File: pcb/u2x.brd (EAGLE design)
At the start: 100 x 100 mm, 9 parts, among them IC4 REG1117, SW20 324_SW, U1 UG-2864HSWEG01, U2 CY8C5868LTI-LP039, U3 USBC_16P

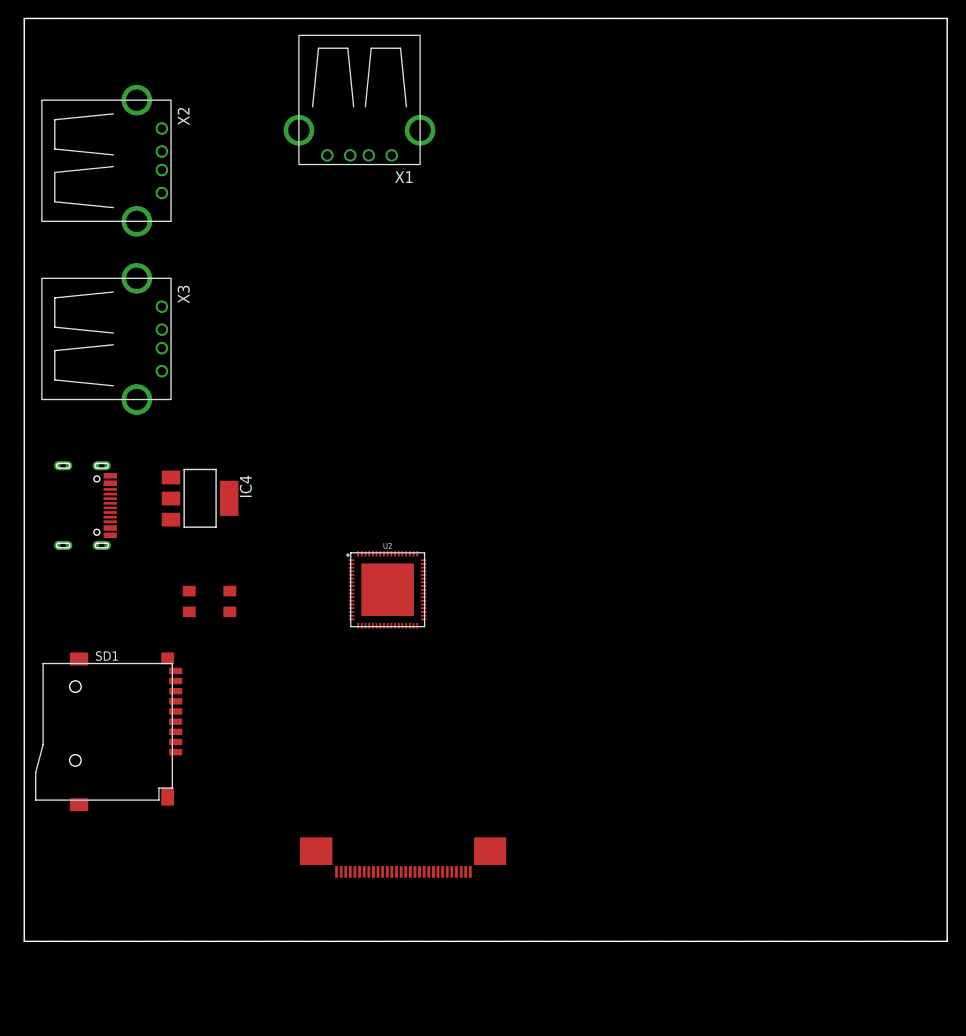
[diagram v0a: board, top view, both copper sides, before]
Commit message: started working on pcb
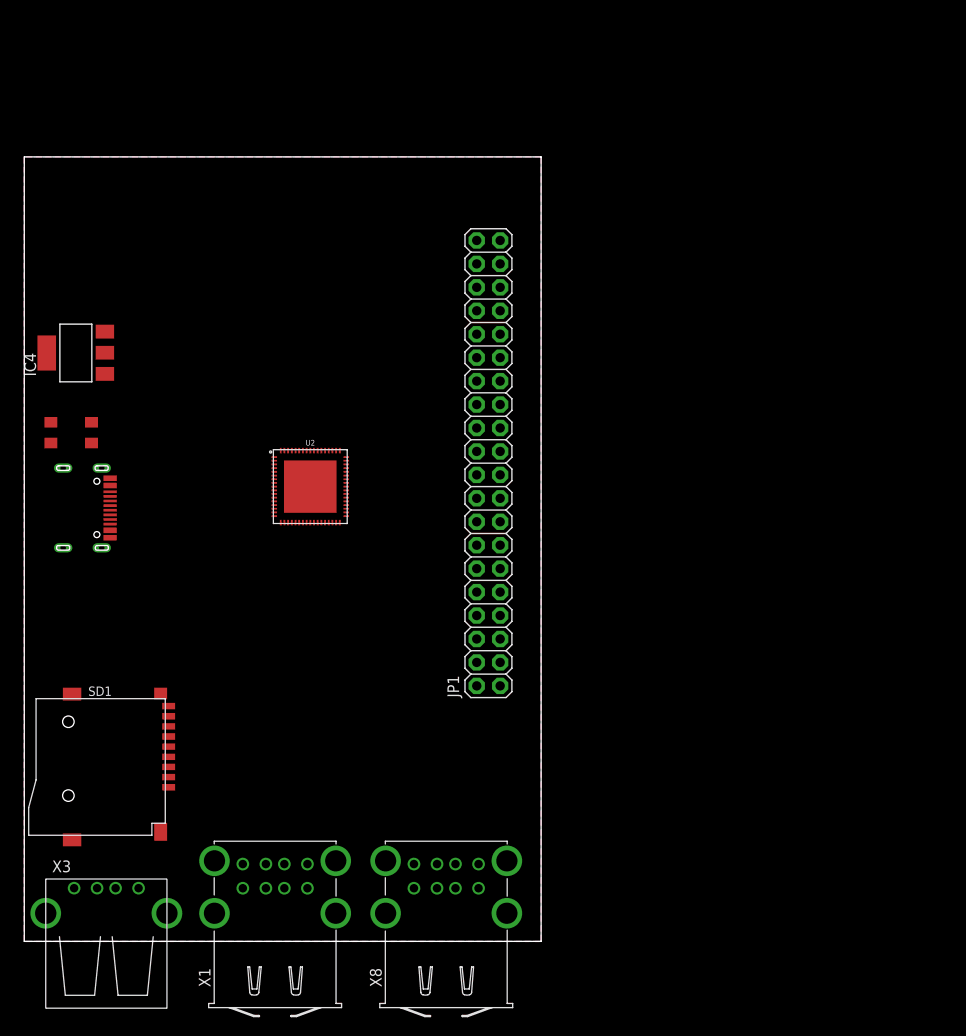
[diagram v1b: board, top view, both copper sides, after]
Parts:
- removed U1: UG-2864HSWEG01, lul:LUL_UG-2864HSWEG01_1.3_WRAPAROUND
- removed X2: (no value), bott:USB-A-H
- added JP1: (no value), adafruit_changed:2X20-BIG
- added X8: USB2, RPB:USB2
- X1: value (none) -> USB2; device bott:USB-A-H -> RPB:USB2
- moved X1 85.3 mm to (27.2, 3.05), turned to 90 degrees
- moved X3 62.3 mm to (8.89, 3.05), turned to 90 degrees
- moved SW20 23.6 mm to (5.08, 55.1)
- moved IC4 20.7 mm to (5.59, 63.8), turned to 90 degrees
- moved U2 14.0 mm to (31.0, 49.3)
- moved SD1 3.89 mm to (8.03, 18.9)
- moved U3 0.25 mm to (5.46, 47.0)
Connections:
- removed net VCC: U1.28
- removed net VLSS: U1.29
- net VDD: no longer U1.9
- net VSS: no longer U1.31, U1.32, U1.8
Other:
- board size 100 x 100 mm -> 56 x 85 mm
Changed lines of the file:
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@@
 <board>
 <plain>
-<wire x1="0" y1="100" x2="0" y2="0" width="0" layer="20"/>
-<wire x1="0" y1="0" x2="100" y2="0" width="0" layer="20"/>
-<wire x1="100" y1="0" x2="100" y2="100" width="0" layer="20"/>
-<wire x1="100" y1="100" x2="0" y2="100" width="0" layer="20"/>
-<rectangle x1="22.4834" y1="56.8782" x2="56.4834" y2="79.8782" layer="51"/>
-<rectangle x1="19.372" y1="28.992" x2="59.372" y2="43.992" layer="51" rot="R90"/>
-<rectangle x1="62.23" y1="40.894" x2="81.83" y2="65.894" layer="51"/>
+<wire x1="0" y1="85" x2="0" y2="0" width="0" layer="20"/>
+<wire x1="0" y1="0" x2="56" y2="0" width="0" layer="20"/>
+<wire x1="56" y1="0" x2="56" y2="85" width="0" layer="20"/>
+<wire x1="56" y1="85" x2="0" y2="85" width="0" layer="20"/>
 </plain>
 <attributes>
@@
 </autorouter>
 <elements>
-<element name="U3" library="my_usbc_16p" package="USBC_16P_FOOT" value="USBC_16P" x="5.461" y="47.2186" smashed="yes" rot="R270"/>
-<element name="U1" library="lul" package="LUL_UG-2864HSWEG01_1.3_WRAPAROUND" value="UG-2864HSWEG01" x="41.0784" y="7.5306" smashed="yes" rot="MR180"/>
-<element name="SD1" library="clock" package="TF-PULL" value="TF-HOLDER" x="8.7884" y="22.7076" smashed="yes" rot="R90">
-<attribute name="NAME" x="7.6884" y="30.4076" size="1.016" layer="25" ratio="18"/>
-</element>
-<element name="IC4" library="clock" package="SOT223" value="REG1117" x="19.05" y="48.006" smashed="yes" rot="R270">
-<attribute name="MF" value="" x="31.75" y="55.626" size="1.778" layer="27" rot="R270" display="off"/>
-<attribute name="MPN" value="REG1117" x="31.75" y="55.626" size="1.778" layer="27" rot="R270" display="off"/>
-<attribute name="NAME" x="23.368" y="50.546" size="1.27" layer="25" ratio="10" rot="R270"/>
-<attribute name="OC_FARNELL" value="1097566" x="31.75" y="55.626" size="1.778" layer="27" rot="R270" display="off"/>
-<attribute name="OC_NEWARK" value="14P6981" x="31.75" y="55.626" size="1.778" layer="27" rot="R270" display="off"/>
-<attribute name="VALUE" x="13.208" y="50.8" size="1.27" layer="27" ratio="10" rot="R270"/>
-</element>
-<element name="SW20" library="3pos_slide_switch_centered" package="342_SWICH_FOOT" value="324_SW" x="20.066" y="36.83" smashed="yes"/>
-<element name="X1" library="bott" package="USB-A-H" value="" x="36.322" y="87.884" smashed="yes" rot="R270">
-<attribute name="NAME" x="40.132" y="82.169" size="1.27" layer="25"/>
-</element>
-<element name="X2" library="bott" package="USB-A-H" value="" x="12.192" y="84.582" smashed="yes">
-<attribute name="NAME" x="17.907" y="88.392" size="1.27" layer="25" rot="R90"/>
-</element>
-<element name="X3" library="bott" package="USB-A-H" value="" x="12.192" y="65.278" smashed="yes">
-<attribute name="NAME" x="17.907" y="69.088" size="1.27" layer="25" rot="R90"/>
-</element>
-<element name="U2" library="SparkFun-IC-Microcontroller" package="QFN-68" value="CY8C5868LTI-LP039" x="39.37" y="38.1" smashed="yes">
-<attribute name="NAME" x="39.37" y="42.545" size="0.6096" layer="25" font="vector" ratio="20" align="bottom-center"/>
-<attribute name="PROD_ID" value="IC-12391" x="39.37" y="38.1" size="1.778" layer="27" display="off"/>
-<attribute name="VALUE" x="39.37" y="33.02" size="0.6096" layer="27" font="vector" ratio="20" align="bottom-center"/>
+<element name="U3" library="my_usbc_16p" package="USBC_16P_FOOT" value="USBC_16P" x="5.461" y="46.9646" smashed="yes" rot="R270"/>
+<element name="SD1" library="clock" package="TF-PULL" value="TF-HOLDER" x="8.0264" y="18.8976" smashed="yes" rot="R90">
+<attribute name="NAME" x="6.9264" y="26.5976" size="1.016" layer="25" ratio="18"/>
+</element>
+<element name="IC4" library="clock" package="SOT223" value="REG1117" x="5.588" y="63.754" smashed="yes" rot="R90">
+<attribute name="MF" value="" x="-7.112" y="56.134" size="1.778" layer="27" rot="R90" display="off"/>
+<attribute name="MPN" value="REG1117" x="-7.112" y="56.134" size="1.778" layer="27" rot="R90" display="off"/>
+<attribute name="NAME" x="1.27" y="61.214" size="1.27" layer="25" ratio="10" rot="R90"/>
+<attribute name="OC_FARNELL" value="1097566" x="-7.112" y="56.134" size="1.778" layer="27" rot="R90" display="off"/>
+<attribute name="OC_NEWARK" value="14P6981" x="-7.112" y="56.134" size="1.778" layer="27" rot="R90" display="off"/>
+<attribute name="VALUE" x="11.43" y="60.96" size="1.27" layer="27" ratio="10" rot="R90"/>
+</element>
+<element name="SW20" library="3pos_slide_switch_centered" package="342_SWICH_FOOT" value="324_SW" x="5.08" y="55.118" smashed="yes"/>
+<element name="X3" library="bott" package="USB-A-H" value="" x="8.89" y="3.048" smashed="yes" rot="R90">
+<attribute name="NAME" x="5.08" y="8.763" size="1.27" layer="25" rot="R180"/>
+</element>
+<element name="U2" library="SparkFun-IC-Microcontroller" package="QFN-68" value="CY8C5868LTI-LP039" x="30.988" y="49.276" smashed="yes">
+<attribute name="NAME" x="30.988" y="53.721" size="0.6096" layer="25" font="vector" ratio="20" align="bottom-center"/>
+<attribute name="PROD_ID" value="IC-12391" x="30.988" y="49.276" size="1.778" layer="27" display="off"/>
+<attribute name="VALUE" x="30.988" y="44.196" size="0.6096" layer="27" font="vector" ratio="20" align="bottom-center"/>
+</element>
+<element name="JP1" library="adafruit_changed" package="2X20-BIG" value="" x="50.292" y="51.816" smashed="yes" rot="R90">
+<attribute name="NAME" x="47.117" y="26.416" size="1.27" layer="25" ratio="10" rot="R90"/>
+<attribute name="VALUE" x="54.737" y="26.416" size="1.27" layer="27" rot="R90"/>
+</element>
+<element name="X8" library="RPB" package="USB2" value="USB2" x="45.72" y="3.048" smashed="yes" rot="R90">
+<attribute name="MF" value="" x="45.72" y="3.048" size="1.778" layer="27" rot="R90" display="off"/>
+<attribute name="MPN" value="" x="45.72" y="3.048" size="1.778" layer="27" rot="R90" display="off"/>
+<attribute name="NAME" x="38.72" y="-4.952" size="1.27" layer="25" rot="R90"/>
+<attribute name="OC_FARNELL" value="unknown" x="45.72" y="3.048" size="1.778" layer="27" rot="R90" display="off"/>
+<attribute name="OC_NEWARK" value="unknown" x="45.72" y="3.048" size="1.778" layer="27" rot="R90" display="off"/>
+<attribute name="VALUE" x="51.22" y="0.048" size="1.27" layer="27" rot="R180"/>
+</element>
+<element name="X1" library="RPB" package="USB2" value="USB2" x="27.178" y="3.048" smashed="yes" rot="R90">
+<attribute name="MF" value="" x="27.178" y="3.048" size="1.778" layer="27" rot="R90" display="off"/>
+<attribute name="MPN" value="" x="27.178" y="3.048" size="1.778" layer="27" rot="R90" display="off"/>
+<attribute name="NAME" x="20.178" y="-4.952" size="1.27" layer="25" rot="R90"/>
+<attribute name="OC_FARNELL" value="unknown" x="27.178" y="3.048" size="1.778" layer="27" rot="R90" display="off"/>
+<attribute name="OC_NEWARK" value="unknown" x="27.178" y="3.048" size="1.778" layer="27" rot="R90" display="off"/>
+<attribute name="VALUE" x="32.678" y="0.048" size="1.27" layer="27" rot="R180"/>
 </element>
 </elements>
@@
 <signal name="GND">
 <polygon width="0.1524" layer="1" isolate="0.254">
-<vertex x="0" y="100"/>
+<vertex x="0" y="85"/>
 <vertex x="0" y="0"/>
-<vertex x="100" y="0"/>
-<vertex x="100" y="100"/>
+<vertex x="56" y="0"/>
+<vertex x="56" y="85"/>
 </polygon>
 <contactref element="IC4" pad="1"/>
@@
 <signal name="+3V3">
 <polygon width="0.1524" layer="16" isolate="0.254">
-<vertex x="0" y="100"/>
-<vertex x="100" y="100"/>
-<vertex x="100" y="0"/>
+<vertex x="0" y="85"/>
+<vertex x="56" y="85"/>
+<vertex x="56" y="0"/>
 <vertex x="0" y="0"/>
 </polygon>
 </signal>
-<signal name="VCC">
-<contactref element="U1" pad="28"/>
-</signal>
 <signal name="VDD">
-<contactref element="U1" pad="9"/>
 <contactref element="SD1" pad="4"/>
-<wire x1="16.4084" y1="23.8076" x2="37.8284" y2="7.5306" width="0" layer="19" extent="1-1"/>
-</signal>
-<signal name="VLSS">
-<contactref element="U1" pad="29"/>
 </signal>
 <signal name="VSS">
-<contactref element="U1" pad="8"/>
-<contactref element="U1" pad="31"/>
-<contactref element="U1" pad="32"/>
 <contactref element="SD1" pad="6"/>
-<wire x1="37.3284" y1="7.5306" x2="50.4784" y2="9.7706" width="0" layer="19" extent="1-1"/>
-<wire x1="31.6284" y1="9.7706" x2="37.3284" y2="7.5306" width="0" layer="19" extent="1-1"/>
-<wire x1="16.4084" y1="26.0076" x2="31.6284" y2="9.7706" width="0" layer="19" extent="1-1"/>
 </signal>
 </signals>
